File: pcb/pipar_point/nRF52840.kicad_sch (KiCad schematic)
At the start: 75 parts, among them J53 Conn_02x04_Odd_Even, P1 USB-C, Q1 AO3416 N-channel MOSFET, SW1 Reset, U1 BQ21040DBVR, U11 BQ24075RGT, U2 nRF52840, U3 ESDR0502NMUTAG, U7 XC6220B331MR, U9 MAX17048, Y1 32.768 kHz, Y2 32MHz

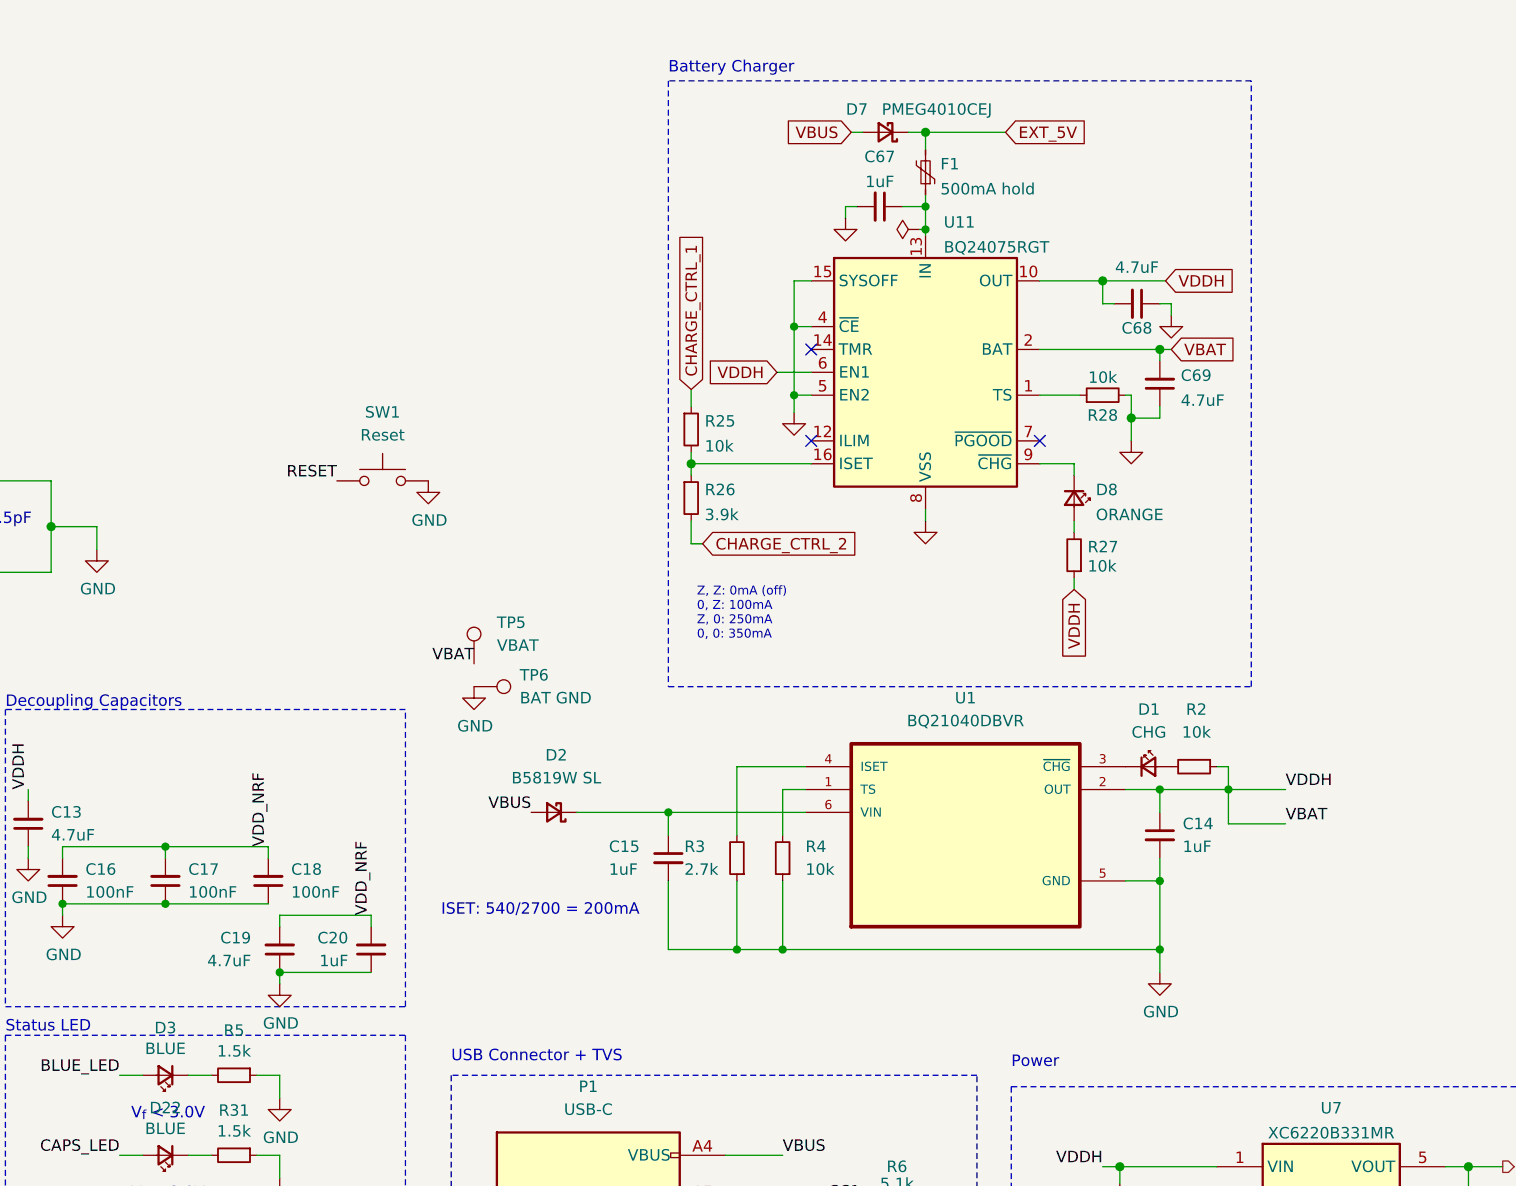
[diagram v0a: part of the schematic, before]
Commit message: more progress on pipar point
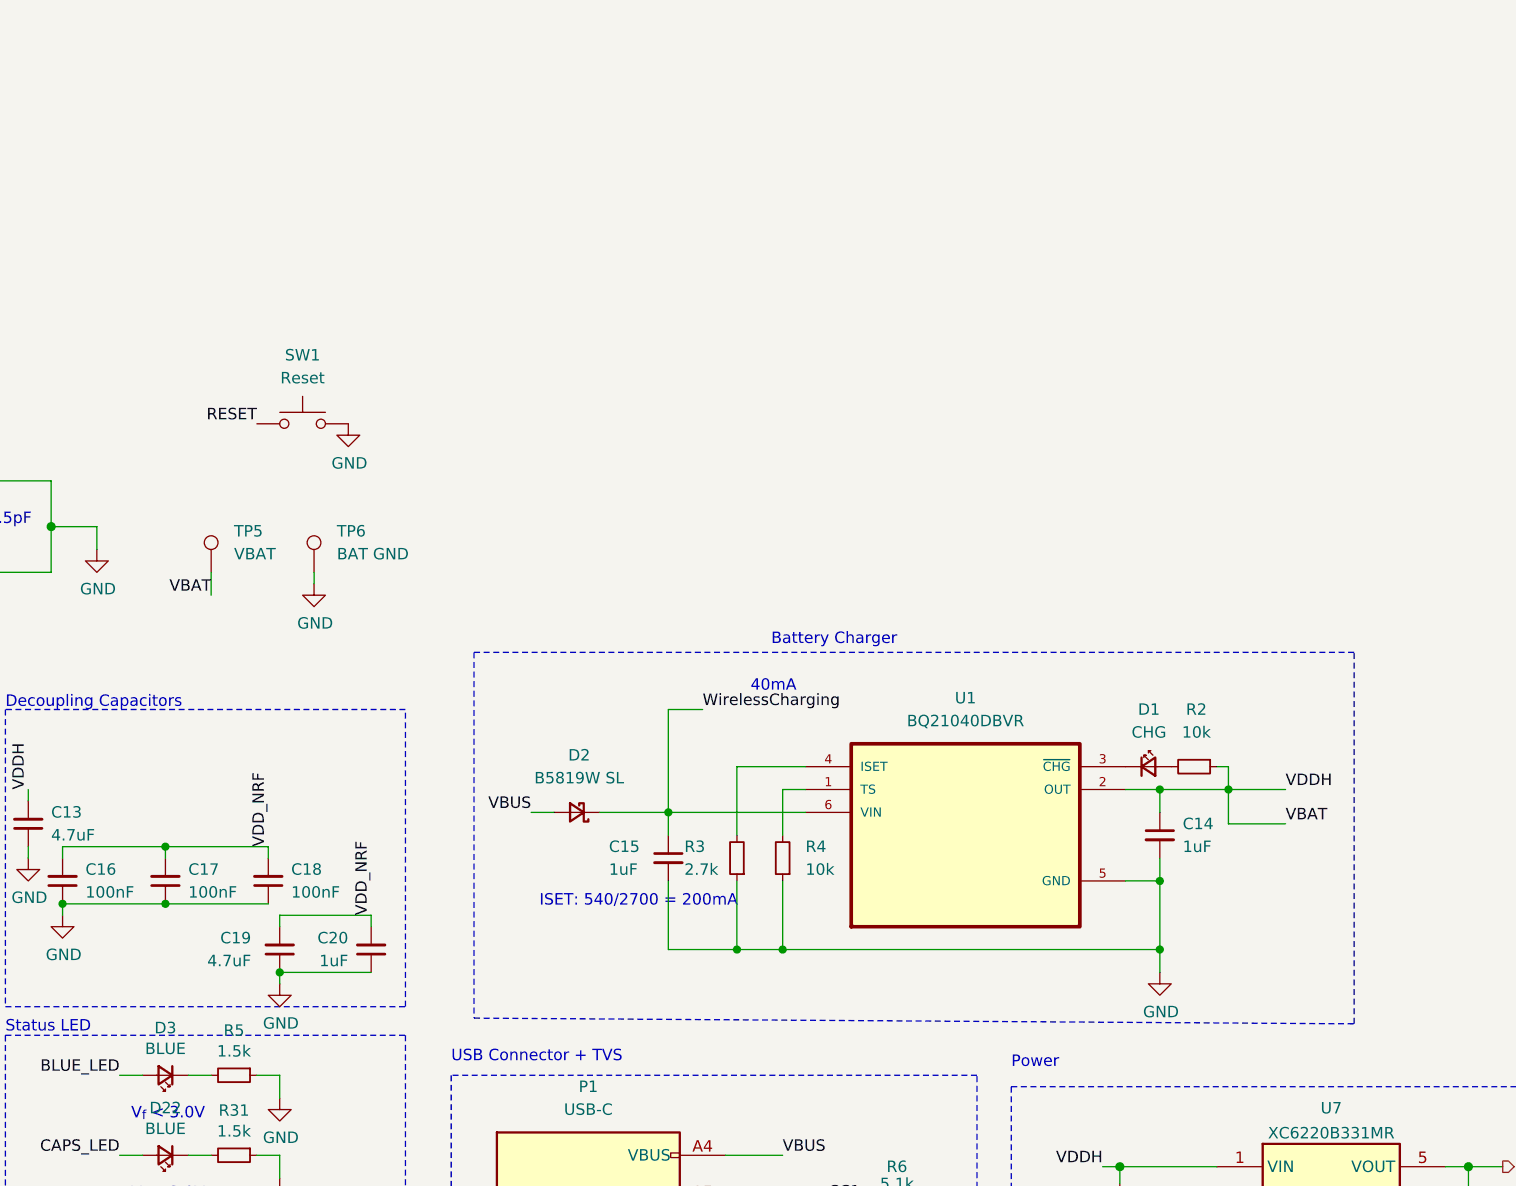
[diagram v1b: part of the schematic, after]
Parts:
- removed C67: 1uF, footprints:Capacitor_0402_1005M-nosilk, symbol Device:C_Small
- removed C68, C69: 4.7uF, footprints:Capacitor_0402_1005M-nosilk, symbol Device:C_Small
- removed D7: PMEG4010CEJ, footprints:D_SOD-323F-nosilk, symbol Device:D_Schottky_Small
- removed D8: ORANGE, footprints:LED_0402_1005Metric-nosilk, symbol Device:LED_Small
- removed F1: 500mA hold, footprints:Fuse_0402_1005Metric, symbol Device:Polyfuse_Small
- removed R25, R27, R28: 10k, footprints:Resistor_0402_1005M-nosilk, symbol Device:R_Small
- removed R26: 3.9k, footprints:Resistor_0402_1005M-nosilk, symbol Device:R_Small
- removed U11: BQ24075RGT, footprints:VQFN-16-1EP_3x3mm_P0.5mm_EP1.6x1.6mm, symbol Battery_Management:BQ24075RGT
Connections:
- net WirelessCharging: now reaches C15.1, D2.1 (K), U1.6 (VIN)
- no-connect marks 26 -> 23
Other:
- note added: "40mA"
- note removed: "Z, Z: 0mA (off) 0, Z: 100mA Z, 0: 250mA 0, 0: 350mA"
- moved on the sheet: D2, SW1, TP5, TP6
